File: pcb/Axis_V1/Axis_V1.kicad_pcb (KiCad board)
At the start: 2 copper layers, 101.6 x 55.9 mm, 35 parts, among them J1 Screw_Terminal_01x03, J10 BOILER_3v3, J11 3WAY_L, J2 Screw_Terminal_01x03, J3 BREW_SW, J4 STEAM_SW, J5 AC_L, J6 AC_N, J7 BOILER_GND, J9 PUMP_L, Q1 BC547, Q2 BT136-500, Q3 BT136-500, U1 Pico, U2 ADS1115IDGS, U3 MAX31855KASA

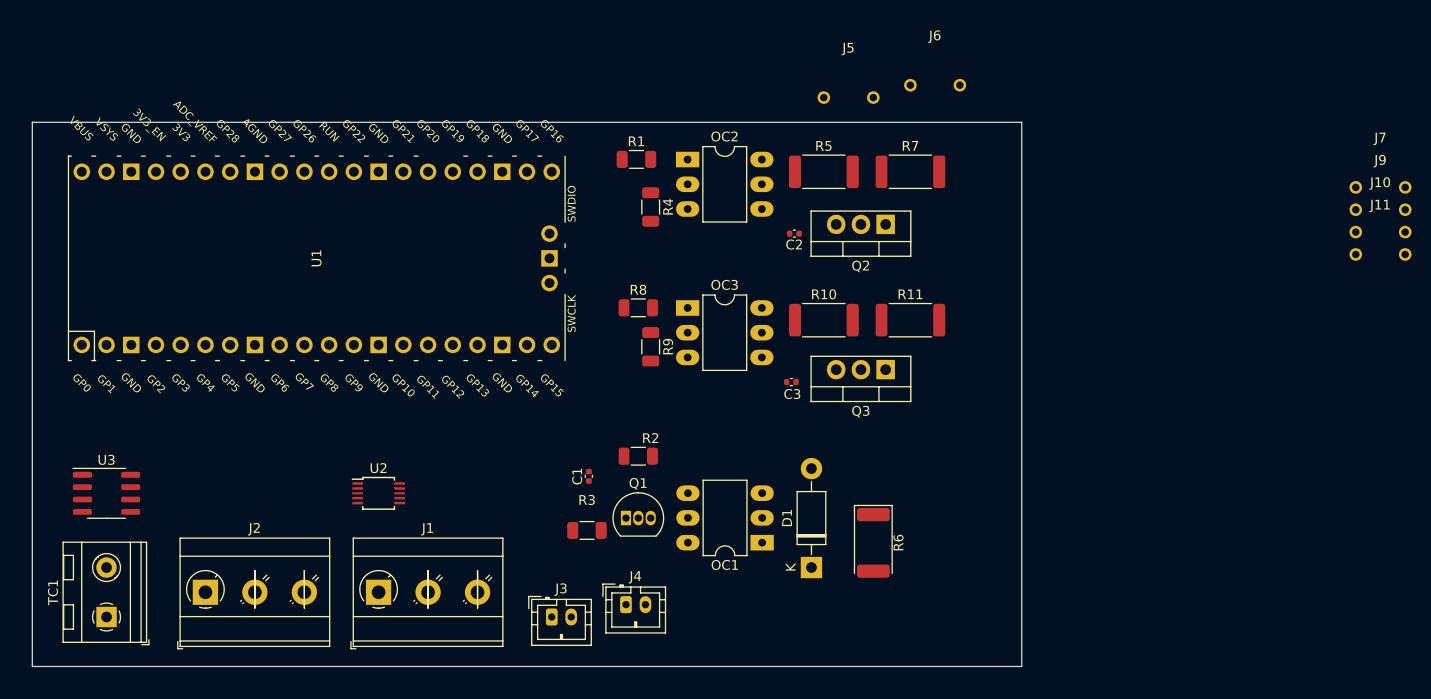
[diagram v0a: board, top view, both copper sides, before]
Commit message: Add more stuff for pcb
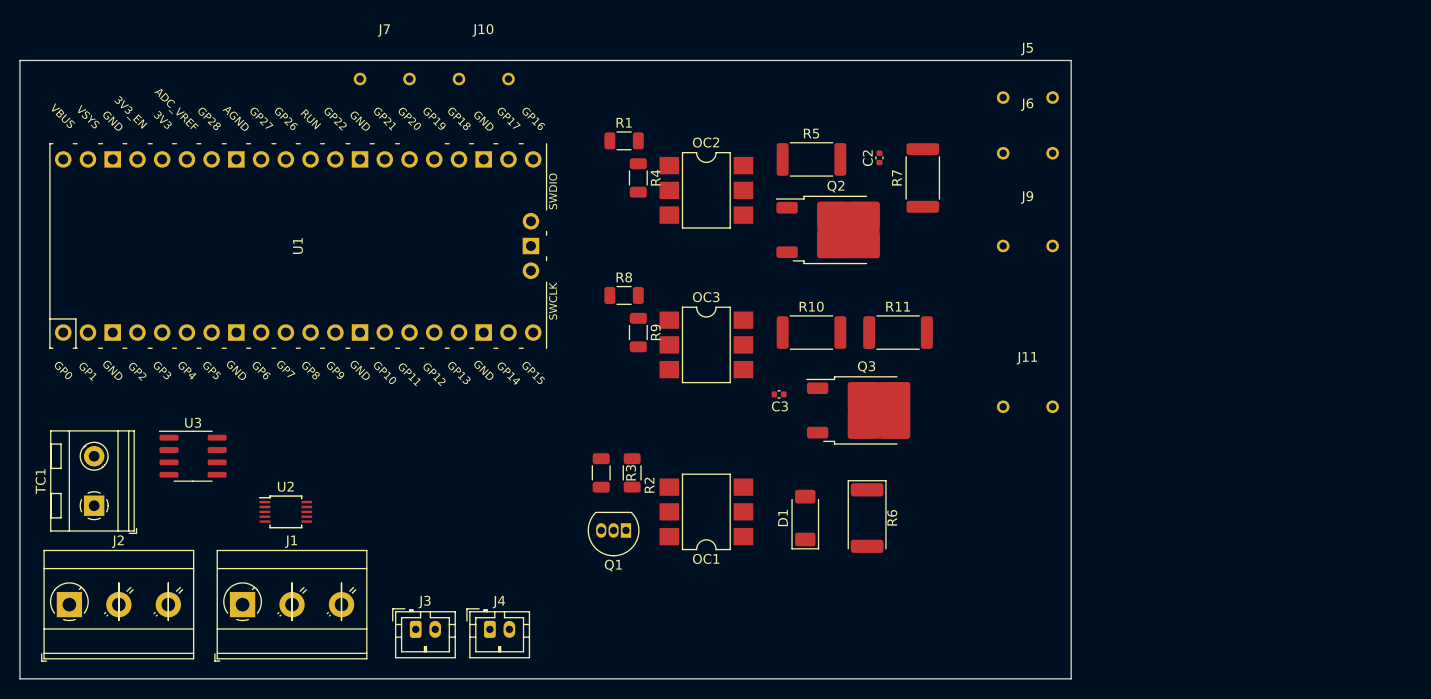
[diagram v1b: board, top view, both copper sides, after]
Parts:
- removed C1: 100nF, Capacitor_SMD:C_0402_1005Metric
- D1: value 1N4001 -> RFN1LAM6STR; footprint Diode_THT:D_DO-41_SOD81_P10.16mm_Horizontal -> Diode_SMD:D_SOD-128
- OC1: footprint Package_DIP:DIP-6_W7.62mm_LongPads -> DIP:SMDIP-6_W7.62mm
- OC2, OC3: value MOC3021M -> MOC3021S-TA1; footprint Package_DIP:DIP-6_W7.62mm_LongPads -> DIP:SMDIP-6_W7.62mm
- Q2, Q3: footprint Package_TO_SOT_THT:TO-220-3_Vertical -> Package_TO_SOT_SMD:TO-252-2
- moved J7 102.9 mm to (145.4, 46.4)
- moved J10 93.4 mm to (155.6, 46.4)
- moved J11 39.4 mm to (211.5, 80.0)
- moved J9 36.4 mm to (211.5, 63.5)
- moved J5 18.4 mm to (211.5, 48.3)
- moved J4 14.2 mm to (156.2, 102.9)
- moved J1 14.0 mm to (130.8, 100.3)
- moved J2 14.0 mm to (113.0, 100.3)
- moved J3 14.0 mm to (148.6, 102.9)
- moved J6 11.8 mm to (211.5, 54.0)
- moved C2 11.7 mm to (196.2, 54.5), turned to 90 degrees
- moved TC1 11.5 mm to (115.6, 90.2)
- moved U2 9.71 mm to (135.3, 90.8)
- moved U3 9.67 mm to (125.7, 85.1)
- moved OC1 6.54 mm to (178.4, 90.8)
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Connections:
- OC1 pad 5: +3.3V -> unconnected-(OC1-Pad5)
- OC1 pad 6: unconnected-(OC1-Pad6) -> +3.3V
- U3 pad 5: PIN_10 -> PIN_12
- U3 pad 7: PIN_12 -> PIN_10
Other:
- board size 101.6 x 55.9 mm -> 108 x 63.5 mm
